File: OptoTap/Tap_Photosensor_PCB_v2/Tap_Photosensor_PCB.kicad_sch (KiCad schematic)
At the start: 10 parts, among them J1 Conn_01x03, U1 OPB961N51, U2 AP63205WU

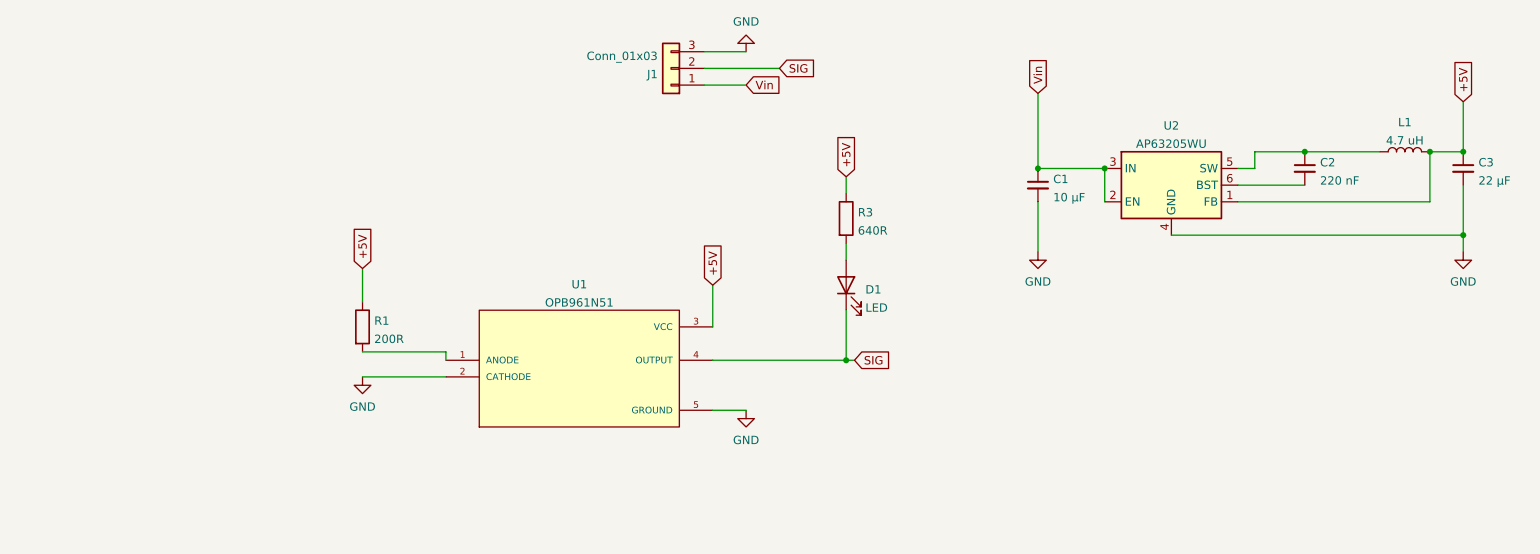
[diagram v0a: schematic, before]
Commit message: updated OptoTap boards
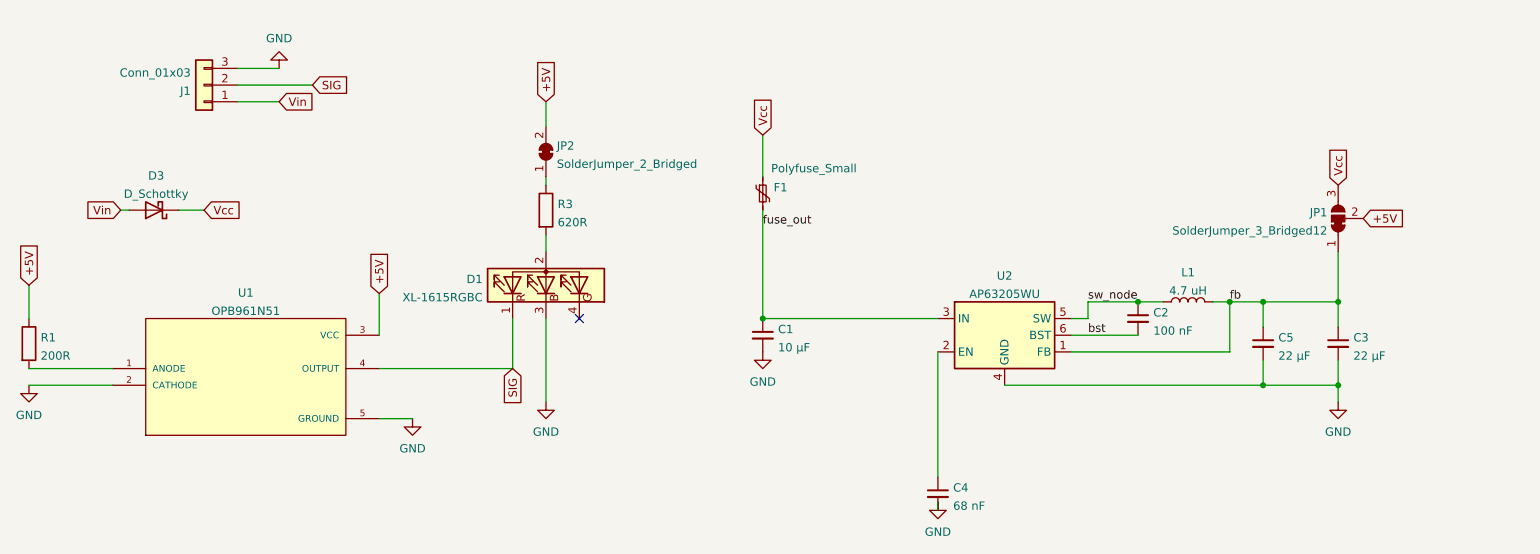
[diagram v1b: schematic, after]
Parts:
- removed D1: LED, LED_SMD:LED_0603_1608Metric, symbol Device:LED
- added C4: 68 nF, Capacitor_SMD:C_0402_1005Metric, symbol Device:C_Small
- added C5: 22 µF, Capacitor_SMD:C_0603_1608Metric, symbol Device:C_Small
- added D1: XL-1615RGBC, LED_SMD:LED_0606_1432, symbol LED:XL-1615RBGC
- added D3: D_Schottky, Diode_SMD:D_SOD-323, symbol Device:D_Schottky
- added F1: Polyfuse_Small, Resistor_SMD:R_0805_2012Metric, symbol Device:Polyfuse_Small
- added JP1: SolderJumper_3_Bridged12, Jumper:SolderJumper-3_P1.3mm_Bridged12_RoundedPad1.0x1.5mm_NumberLabels, symbol Jumper:SolderJumper_3_Bridged12
- added JP2: SolderJumper_2_Bridged, Jumper:SolderJumper-2_DARKMODE, symbol Jumper:SolderJumper_2_Bridged
- C1: LCSC (none) -> C440198; PARTNUM (none) -> GRM21BR61H106KE43L
- C2: value 220 nF -> 100 nF; footprint Capacitor_SMD:C_0805_2012Metric -> Capacitor_SMD:C_0402_1005Metric; LCSC (none) -> C307331; PARTNUM (none) -> CL05B104KB54PNC
- C3: footprint Capacitor_SMD:C_0805_2012Metric -> Capacitor_SMD:C_0603_1608Metric; LCSC (none) -> C84419; PARTNUM (none) -> GRM188R61A226ME15D
- L1: footprint Inductor_SMD:L_0805_2012Metric -> Inductor_SMD:CKCS3010; LCSC (none) -> C354557; PARTNUM (none) -> CKCS3012-4.7uH/M
- R1: LCSC (none) -> C8218; PARTNUM (none) -> 0603WAF2000T5E
- R3: value 640R -> 620R; LCSC (none) -> C23220; PARTNUM (none) -> 0603WAF6200T5E
- U1: footprint OPTO_OPB961N51 -> footprints:OPTO_EE-SX398_OPB666N
- U2: LCSC (none) -> C2071056; PARTNUM (none) -> AP63205WU
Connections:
- net +5V: now also JP1.2 (C), JP2.2 (B); no longer C3.1, L1.2, R3.1, U2.1 (FB)
- net GND: now also C4.2, C5.2, D1.3 (B)
- net SIG: now also D1.1 (R)
- net Vin: now also D3.2 (A); no longer C1.1, U2.2 (EN), U2.3 (IN)
- net at R3.2: now also D1.2 (A)
- net sw_node: now reaches C2.1, L1.1, U2.5 (SW)
- net bst: now reaches C2.2, U2.6 (BST)
- new net: C4.1, U2.2 (EN)
- new net: JP2.1 (A), R3.1
- new net Vcc: D3.1 (K), F1.1, JP1.3 (B)
- new net fb: C3.1, C5.1, JP1.1 (A), L1.2, U2.1 (FB)
- new net fuse_out: C1.1, F1.2, U2.3 (IN)
- no-connect marks 0 -> 1
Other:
- moved on the sheet: C1, C2, C3, J1, L1, R1, R3, U1, U2
